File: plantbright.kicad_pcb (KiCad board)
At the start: 2 copper layers, 33 x 54 mm, 23 parts, among them J1 POWER OUT, J2 USB-C, Q1 AO3400A, Q2 AO3400A, Q3 AO3400A, Q5 AO3400A, SW1 USER 0, U1 XIAO-ESP32-C6

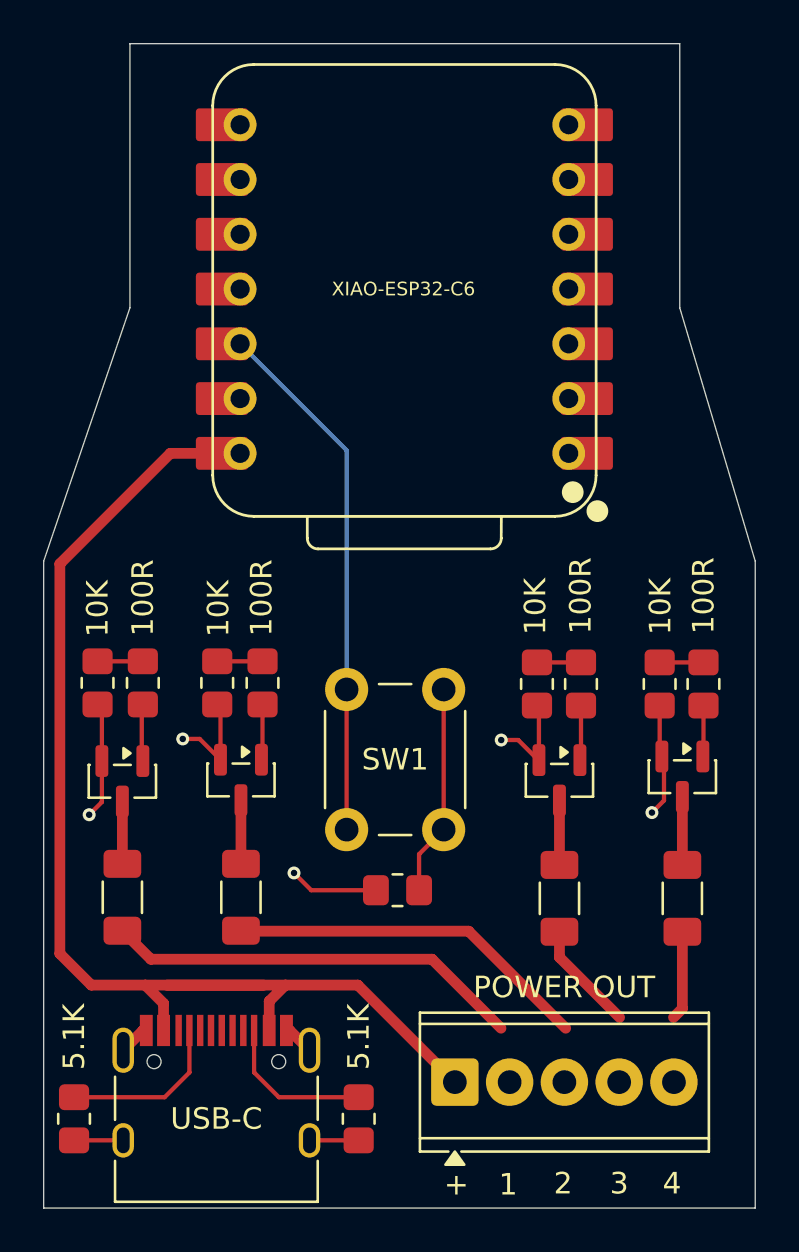
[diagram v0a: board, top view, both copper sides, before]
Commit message: Add cap
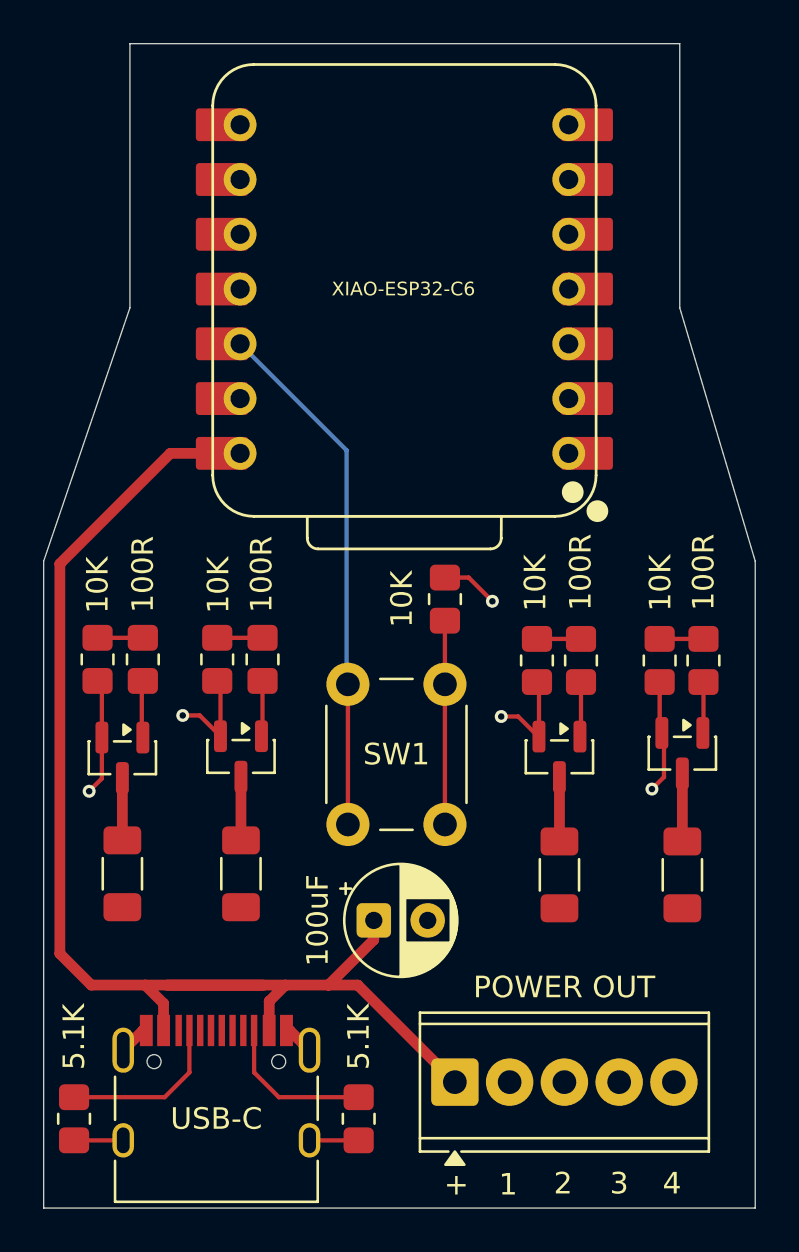
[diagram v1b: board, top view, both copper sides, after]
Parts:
- added C1: 100uF, Capacitor_THT:CP_Radial_D5.0mm_P2.50mm, F.Cu at (152.1, 105.0)
- moved R9 13.7 mm to (155.4, 90.1), turned to 90 degrees
- moved Q1 1.09 mm to (166.4, 97.2)
- moved Q2 1.09 mm to (160.7, 97.4)
- moved R1 1.09 mm to (167.4, 92.9)
- moved R10 1.09 mm to (166.4, 102.9)
- moved R11 1.09 mm to (160.7, 102.9)
- moved R12 1.09 mm to (145.9, 102.8)
- moved R13 1.09 mm to (140.4, 102.8)
- moved R2 1.09 mm to (165.4, 92.9)
- moved R3 1.09 mm to (161.7, 92.9)
- moved R4 1.09 mm to (159.7, 92.9)
- moved Q3 1.09 mm to (145.9, 97.4)
- moved Q5 1.09 mm to (140.4, 97.5)
- moved R5 1.09 mm to (146.9, 92.9)
- moved R6 1.09 mm to (144.8, 92.9)
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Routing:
- net Net-(J1-Pin_5): track 19.4 -> 0.00 mm
- net Net-(J1-Pin_4): track 16.9 -> 0.03 mm
- net Net-(J1-Pin_3): track 5.13 -> 0.00 mm
- net Net-(J1-Pin_2): track 4.14 -> 0.00 mm
- net +5V: track 58.6 -> 62.5 mm
- net GND: track 31.7 -> 30.2 mm
